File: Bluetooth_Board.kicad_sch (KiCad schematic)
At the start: 0 parts

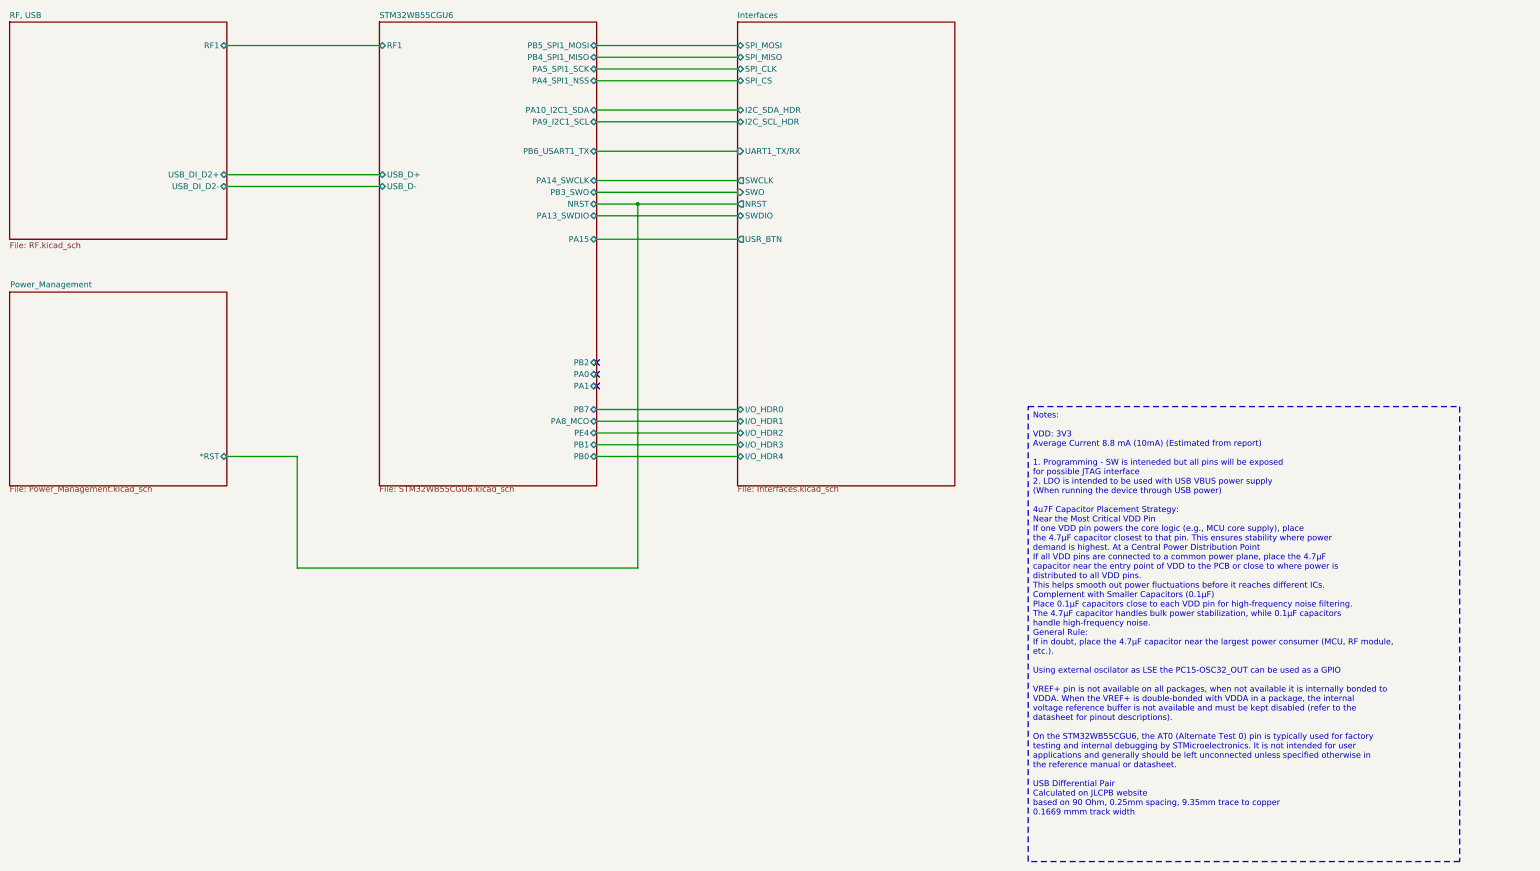
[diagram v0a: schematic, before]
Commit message: JLCPCB Check
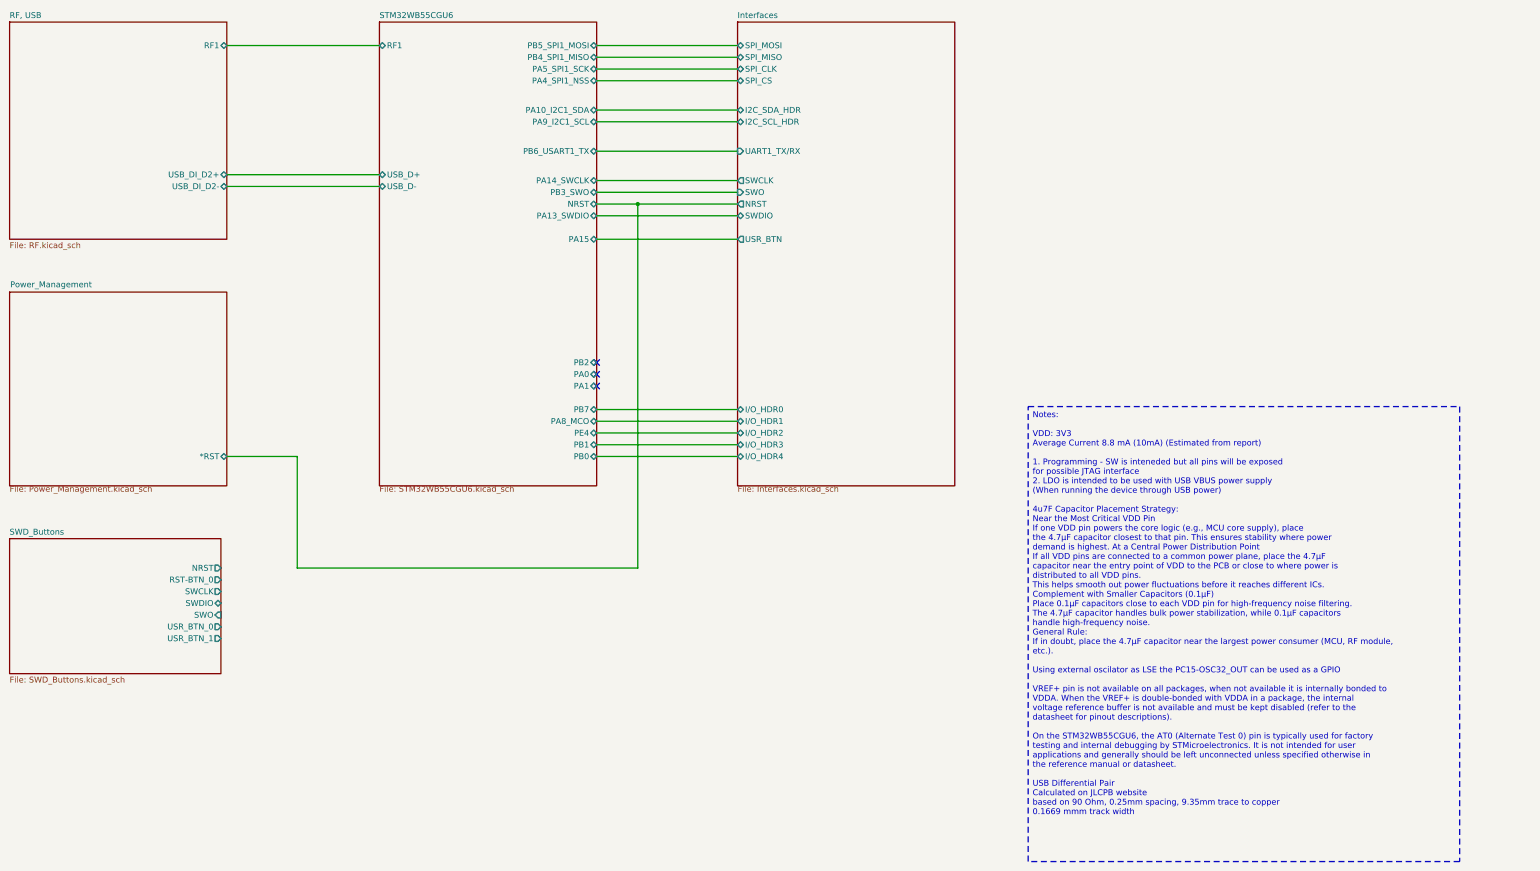
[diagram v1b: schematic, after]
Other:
- added sheet SWD_Buttons (SWD_Buttons.kicad_sch)
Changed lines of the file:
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@@
 (kicad_sch
-	(version 20231120)
+	(version 20260306)
 	(generator "eeschema")
-	(generator_version "8.0")
+	(generator_version "10.0")
 	(paper "USLetter")
 	(title_block
@@
 		(company "Peter Hancak")
 	)
+	(text_box "Notes:\n\nVDD: 3V3\nAverage Current 8.8 mA (10mA) (Estimated from report)\n\n1. Programming - SW is inteneded but all pins will be exposed \nfor possible JTAG interface\n2. LDO is intended to be used with USB VBUS power supply\n   (When running the device through USB power)\n\n4u7F Capacitor Placement Strategy:\nNear the Most Critical VDD Pin\nIf one VDD pin powers the core logic (e.g., MCU core supply), place \nthe 4.7µF capacitor closest to that pin. This ensures stability where power \ndemand is highest. At a Central Power Distribution Point\nIf all VDD pins are connected to a common power plane, place the 4.7µF \ncapacitor near the entry point of VDD to the PCB or close to where power is \ndistributed to all VDD pins.\nThis helps smooth out power fluctuations before it reaches different ICs.\nComplement with Smaller Capacitors (0.1µF)\nPlace 0.1µF capacitors close to each VDD pin for high-frequency noise filtering.\nThe 4.7µF capacitor handles bulk power stabilization, while 0.1µF capacitors \nhandle high-frequency noise.\nGeneral Rule:\nIf in doubt, place the 4.7µF capacitor near the largest power consumer (MCU, RF module, etc.).\n\nUsing external oscilator as LSE the PC15-OSC32_OUT can be used as a GPIO\n\nVREF+ pin is not available on all packages, when not available it is internally bonded to\nVDDA. When the VREF+ is double-bonded with VDDA in a package, the internal\nvoltage reference buffer is not available and must be kept disabled (refer to the\ndatasheet for pinout descriptions).\n\nOn the STM32WB55CGU6, the AT0 (Alternate Test 0) pin is typically used for factory\ntesting and internal debugging by STMicroelectronics. It is not intended for user \napplications and generally should be left unconnected unless specified otherwise in \nthe reference manual or datasheet.\n\nUSB Differential Pair\nCalculated on JLCPB website\nbased on 90 Ohm, 0.25mm spacing, 9.35mm trace to copper\n0.1669 mmm track width"
+		(exclude_from_sim no)
+		(at 257.175 121.285 0)
+		(size 93.345 98.425)
+		(margins 0.9525 0.9525 0.9525 0.9525)
+		(stroke
+			(width 0)
+			(type dash)
+		)
+		(fill
+			(type none)
+		)
+		(effects
+			(font
+				(size 1.27 1.27)
+			)
+			(justify left top)
+		)
+	)
 	(junction
 		(at 172.72 77.47)
@@
 		)
 	)
-	(text_box "Notes:\n\nVDD: 3V3\nAverage Current 8.8 mA (10mA) (Estimated from report)\n\n1. Programming - SW is inteneded but all pins will be exposed \nfor possible JTAG interface\n2. LDO is intended to be used with USB VBUS power supply\n   (When running the device through USB power)\n\n4u7F Capacitor Placement Strategy:\nNear the Most Critical VDD Pin\nIf one VDD pin powers the core logic (e.g., MCU core supply), place \nthe 4.7µF capacitor closest to that pin. This ensures stability where power \ndemand is highest. At a Central Power Distribution Point\nIf all VDD pins are connected to a common power plane, place the 4.7µF \ncapacitor near the entry point of VDD to the PCB or close to where power is \ndistributed to all VDD pins.\nThis helps smooth out power fluctuations before it reaches different ICs.\nComplement with Smaller Capacitors (0.1µF)\nPlace 0.1µF capacitors close to each VDD pin for high-frequency noise filtering.\nThe 4.7µF capacitor handles bulk power stabilization, while 0.1µF capacitors \nhandle high-frequency noise.\nGeneral Rule:\nIf in doubt, place the 4.7µF capacitor near the largest power consumer (MCU, RF module, etc.).\n\nUsing external oscilator as LSE the PC15-OSC32_OUT can be used as a GPIO\n\nVREF+ pin is not available on all packages, when not available it is internally bonded to\nVDDA. When the VREF+ is double-bonded with VDDA in a package, the internal\nvoltage reference buffer is not available and must be kept disabled (refer to the\ndatasheet for pinout descriptions).\n\nOn the STM32WB55CGU6, the AT0 (Alternate Test 0) pin is typically used for factory\ntesting and internal debugging by STMicroelectronics. It is not intended for user \napplications and generally should be left unconnected unless specified otherwise in \nthe reference manual or datasheet.\n\nUSB Differential Pair\nCalculated on JLCPB website\nbased on 90 Ohm, 0.25mm spacing, 9.35mm trace to copper\n0.1669 mmm track width"
-		(exclude_from_sim no)
-		(at 257.175 121.285 0)
-		(size 93.345 98.425)
-		(stroke
-			(width 0)
-			(type dash)
-		)
-		(fill
-			(type none)
-		)
-		(effects
-			(font
-				(size 1.27 1.27)
-			)
-			(justify left top)
-		)
-	)
 	(sheet
 		(at 36.83 38.1)
 		(size 46.99 46.99)
+		(exclude_from_sim no)
+		(in_bom yes)
+		(on_board yes)
+		(dnp no)
 		(fields_autoplaced yes)
 		(stroke
@@
 		)
 		(fill
-			(color 0 255 255 1.0000)
+			(color 0 255 255 1)
 		)
 		(property "Sheetname" "RF, USB"
 			(at 36.83 37.3884 0)
+			(show_name no)
+			(do_not_autoplace no)
 			(effects
 				(font
@@
 		(property "Sheetfile" "RF.kicad_sch"
 			(at 36.83 85.6746 0)
+			(show_name no)
+			(do_not_autoplace no)
 			(effects
 				(font
@@
 	)
 	(sheet
+		(at 36.83 149.86)
+		(size 45.72 29.21)
+		(exclude_from_sim no)
+		(in_bom yes)
+		(on_board yes)
+		(dnp no)
+		(fields_autoplaced yes)
+		(stroke
+			(width 0.1524)
+			(type solid)
+		)
+		(fill
+			(color 0 255 255 1)
+		)
+		(property "Sheetname" "SWD_Buttons"
+			(at 36.83 149.1484 0)
+			(show_name no)
+			(do_not_autoplace no)
+			(effects
+				(font
+					(size 1.27 1.27)
+				)
+				(justify left bottom)
+			)
+		)
+		(property "Sheetfile" "SWD_Buttons.kicad_sch"
+			(at 36.83 179.6546 0)
+			(show_name no)
+			(do_not_autoplace no)
+			(effects
+				(font
+					(size 1.27 1.27)
+				)
+				(justify left top)
+			)
+		)
+		(pin "NRST" output
+			(at 82.55 156.21 0)
+			(effects
+				(font
+					(size 1.27 1.27)
+				)
+				(justify right)
+			)
+		)
+		(pin "RST-BTN_0" output
+			(at 82.55 158.75 0)
+			(effects
+				(font
+					(size 1.27 1.27)
+				)
+				(justify right)
+			)
+		)
+		(pin "SWCLK" output
+			(at 82.55 161.29 0)
+			(effects
+				(font
+					(size 1.27 1.27)
+				)
+				(justify right)
+			)
+		)
+		(pin "SWDIO" bidirectional
+			(at 82.55 163.83 0)
+			(effects
+				(font
+					(size 1.27 1.27)
+				)
+				(justify right)
+			)
+		)
+		(pin "SWO" input
+			(at 82.55 166.37 0)
+			(effects
+				(font
+					(size 1.27 1.27)
+				)
+				(justify right)
+			)
+		)
+		(pin "USR_BTN_0" output
+			(at 82.55 168.91 0)
+			(effects
+				(font
+					(size 1.27 1.27)
+				)
+				(justify right)
+			)
+		)
+		(pin "USR_BTN_1" output
+			(at 82.55 171.45 0)
+			(effects
+				(font
+					(size 1.27 1.27)
+				)
+				(justify right)
+			)
+		)
+		(instances
+			(project "Bluetooth_Board"
+				(path "/05989bb3-969e-4aaa-b344-5f0e2d5af968"
+					(page "6")
+				)
+			)
+		)
+	)
+	(sheet
 		(at 36.83 96.52)
 		(size 46.99 41.91)
+		(exclude_from_sim no)
+		(in_bom yes)
+		(on_board yes)
+		(dnp no)
 		(stroke
 			(width 0.1524)
@@
 		)
 		(fill
-			(color 0 255 255 1.0000)
+			(color 0 255 255 1)
 		)
 		(property "Sheetname" "Power_Management"
 			(at 36.957 95.631 0)
+			(show_name no)
+			(do_not_autoplace no)
 			(effects
 				(font
@@
 		(property "Sheetfile" "Power_Management.kicad_sch"
 			(at 36.83 138.3796 0)
+			(show_name no)
+			(do_not_autoplace no)
 			(effects
 				(font
@@
 		(at 116.84 38.1)
 		(size 46.99 100.33)
+		(exclude_from_sim no)
+		(in_bom yes)
+		(on_board yes)
+		(dnp no)
 		(fields_autoplaced yes)
 		(stroke
@@
 		)
 		(fill
-			(color 0 255 255 1.0000)
+			(color 0 255 255 1)
 		)
 		(property "Sheetname" "STM32WB55CGU6"
 			(at 116.84 37.3884 0)
+			(show_name no)
+			(do_not_autoplace no)
 			(effects
 				(font
@@
 		(property "Sheetfile" "STM32WB55CGU6.kicad_sch"
 			(at 116.84 138.3796 0)
+			(show_name no)
+			(do_not_autoplace no)
 			(effects
 				(font
@@
 		(at 194.31 38.1)
 		(size 46.99 100.33)
+		(exclude_from_sim no)
+		(in_bom yes)
+		(on_board yes)
+		(dnp no)
 		(fields_autoplaced yes)
 		(stroke
@@
 		)
 		(fill
-			(color 0 255 255 1.0000)
+			(color 0 255 255 1)
 		)
 		(property "Sheetname" "Interfaces"
 			(at 194.31 37.3884 0)
+			(show_name no)
+			(do_not_autoplace no)
 			(effects
 				(font
@@
 		(property "Sheetfile" "Interfaces.kicad_sch"
 			(at 194.31 138.3796 0)
+			(show_name no)
+			(do_not_autoplace no)
 			(effects
 				(font
@@
 		)
 	)
+	(embedded_fonts no)
 )
